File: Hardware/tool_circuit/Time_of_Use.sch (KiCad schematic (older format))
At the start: 4 parts

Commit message: Latest revisions to schematic
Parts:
- removed LED1: 151034BS03000, LED_BS03000_WRE, symbol 2021-09-28_17-07-40:151034BS03000
- removed R4: RMCF1206JT150R, RESC3216X70N, symbol RMCF1206JT150R:RMCF1206JT150R
- removed R7: RC1206JR-07110RL, RESC3116X65N, symbol RC1206JR-07110RL:RC1206JR-07110RL
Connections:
- net labels removed: GND, GPIO22
- wire segments 14 -> 6
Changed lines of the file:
@@
 	1    0    0    -1
 $EndComp
-$Comp
-L power:GND #PWR06
-U 1 1 614A4174
-P 4950 5050
-F 0 "#PWR06" H 4950 4800 50  0001 C CNN
-F 1 "GND" H 4955 4877 50  0000 C CNN
-F 2 "" H 4950 5050 50  0001 C CNN
-F 3 "" H 4950 5050 50  0001 C CNN
-	1    4950 5050
-	1    0    0    -1
-$EndComp
-$Comp
-L RMCF1206JT150R:RMCF1206JT150R R4
-U 1 1 614C1CF4
-P 4950 4650
-F 0 "R4" V 4904 4755 50  0000 L CNN
-F 1 "RMCF1206JT150R" V 4995 4755 50  0000 L CNN
-F 2 "RESC3216X70N" H 4950 4650 50  0001 L BNN
-F 3 "" H 4950 4650 50  0001 L BNN
-	1    4950 4650
-	0    1    1    0
-$EndComp
-Wire Wire Line
-	4950 4150 4950 4250
-Connection ~ 4950 4150
 Wire Wire Line
 	6650 4000 6150 4000
-Wire Wire Line
-	6650 3500 6650 3650
-Wire Wire Line
-	3950 4150 4950 4150
 Text Label 4150 4150 0    50   ~ 0
 GPIO17
@@
 Wire Bus Line
 	3650 3900 3850 3900
-$Comp
-L 2021-09-28_17-07-40:151034BS03000 LED1
-U 1 1 615638DB
-P 7200 4000
-F 0 "LED1" V 7347 4228 60  0000 L CNN
-F 1 "151034BS03000" V 7453 4228 60  0000 L CNN
-F 2 "LED_BS03000_WRE" H 7400 3640 60  0001 C CNN
-F 3 "" H 7200 4000 60  0000 C CNN
-	1    7200 4000
-	0    1    1    0
-$EndComp
-Wire Wire Line
-	6650 3650 7200 3650
-Wire Wire Line
-	7200 3650 7200 4000
-Connection ~ 6650 3650
-Wire Wire Line
-	6650 3650 6650 4000
-$Comp
-L RC1206JR-07110RL:RC1206JR-07110RL R7
-U 1 1 6156637C
-P 7200 4800
-F 0 "R7" V 7154 4905 50  0000 L CNN
-F 1 "RC1206JR-07110RL" V 7245 4905 50  0000 L CNN
-F 2 "RESC3116X65N" H 7200 4800 50  0001 L BNN
-F 3 "" H 7200 4800 50  0001 L BNN
-	1    7200 4800
-	0    1    1    0
-$EndComp
-Entry Wire Line
-	3850 4200 3950 4300
-Wire Wire Line
-	3950 4300 3950 5450
-Wire Wire Line
-	3950 5450 7200 5450
-Text Label 3950 4550 0    50   ~ 0
-GPIO22
 $Comp
 L 1825255-1:1825255-1 S1
@@
 $EndComp
 Wire Wire Line
-	7200 5450 7200 5200
-Wire Wire Line
-	4950 4150 5400 4150
-Wire Wire Line
 	6150 4000 6150 3850
 Wire Wire Line
@@
 	5400 3850 5400 4050
 NoConn ~ 5400 4250
-Wire Bus Line
-	3850 3900 3850 4350
 Text HLabel 3650 3900 0    50   BiDi ~ 0
 TIME_OF_USE_DATA
+Wire Wire Line
+	3950 4150 5400 4150
+Wire Wire Line
+	6650 3500 6650 4000
+Wire Bus Line
+	3850 3900 3850 4050
 $EndSCHEMATC

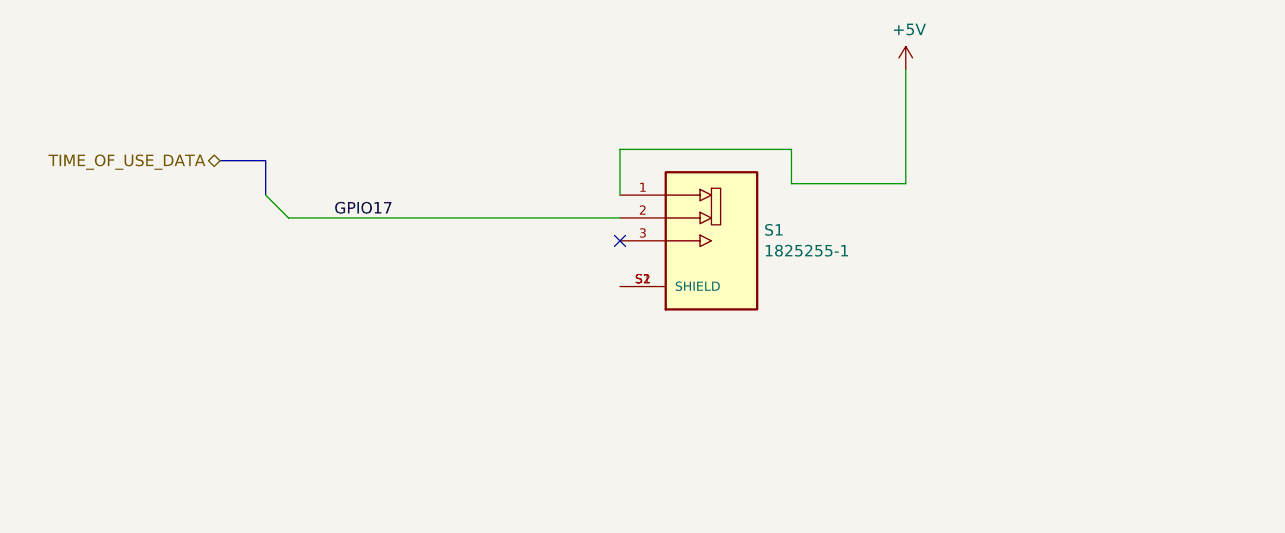
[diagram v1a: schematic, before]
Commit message: udpated circuit
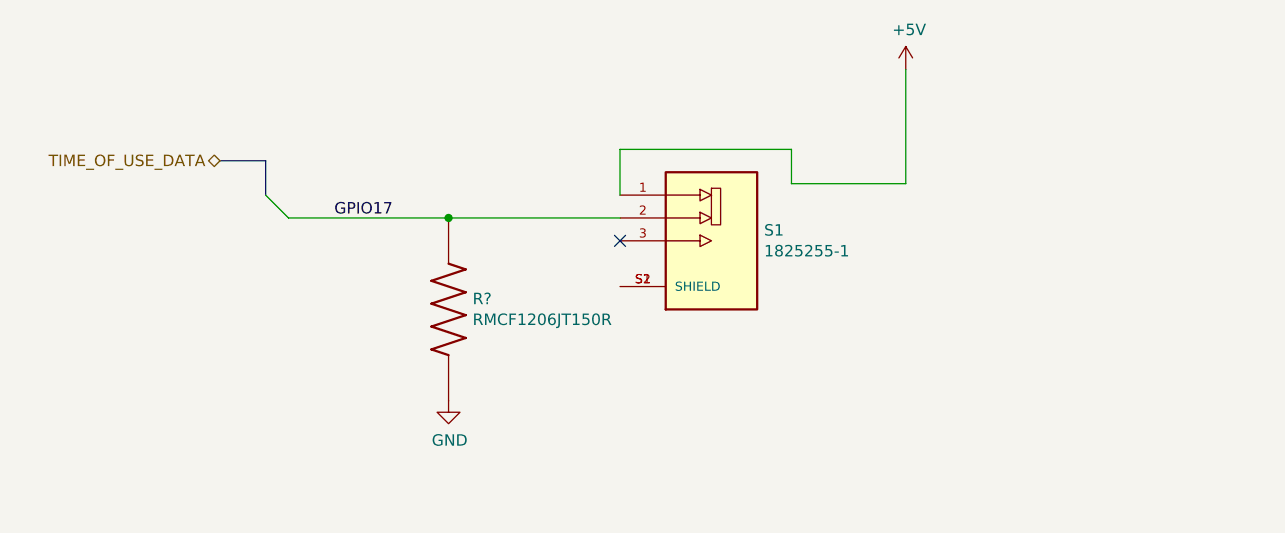
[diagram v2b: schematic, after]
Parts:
- added R?: RMCF1206JT150R, RESC3216X70N, symbol RMCF1206JT150R:RMCF1206JT150R
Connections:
- net GPIO17: now also R?.1
- new net GND: R?.2
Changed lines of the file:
@@
 TIME_OF_USE_DATA
 Wire Wire Line
-	3950 4150 5400 4150
+	3950 4150 4650 4150
 Wire Wire Line
 	6650 3500 6650 4000
 Wire Bus Line
 	3850 3900 3850 4050
+$Comp
+L RMCF1206JT150R:RMCF1206JT150R R?
+U 1 1 61705C6B
+P 4650 4550
+F 0 "R?" V 4604 4655 50  0000 L CNN
+F 1 "RMCF1206JT150R" V 4695 4655 50  0000 L CNN
+F 2 "RESC3216X70N" H 4650 4550 50  0001 L BNN
+F 3 "" H 4650 4550 50  0001 L BNN
+	1    4650 4550
+	0    1    1    0
+$EndComp
+Connection ~ 4650 4150
+Wire Wire Line
+	4650 4150 5400 4150
+$Comp
+L power:GND #PWR?
+U 1 1 61707039
+P 4650 4950
+F 0 "#PWR?" H 4650 4700 50  0001 C CNN
+F 1 "GND" H 4655 4777 50  0000 C CNN
+F 2 "" H 4650 4950 50  0001 C CNN
+F 3 "" H 4650 4950 50  0001 C CNN
+	1    4650 4950
+	1    0    0    -1
+$EndComp
 $EndSCHEMATC
